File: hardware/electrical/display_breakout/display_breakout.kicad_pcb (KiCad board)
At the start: 2 copper layers, 4 parts, among them J1 Conn_02x10_Odd_Even, SW1 RotaryEncoder_Switch, SW2 SW_Push, SW3 SW_Push

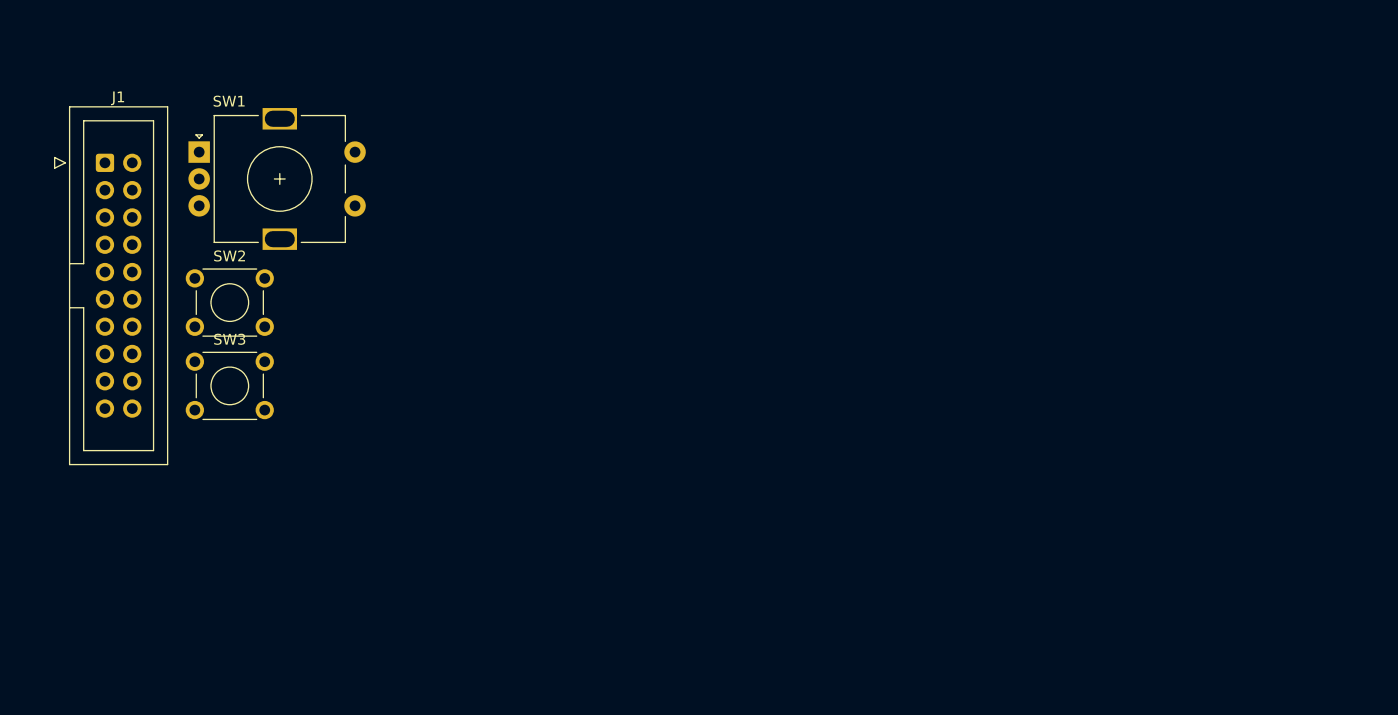
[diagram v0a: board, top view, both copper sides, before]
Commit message: updated schematic to latest version
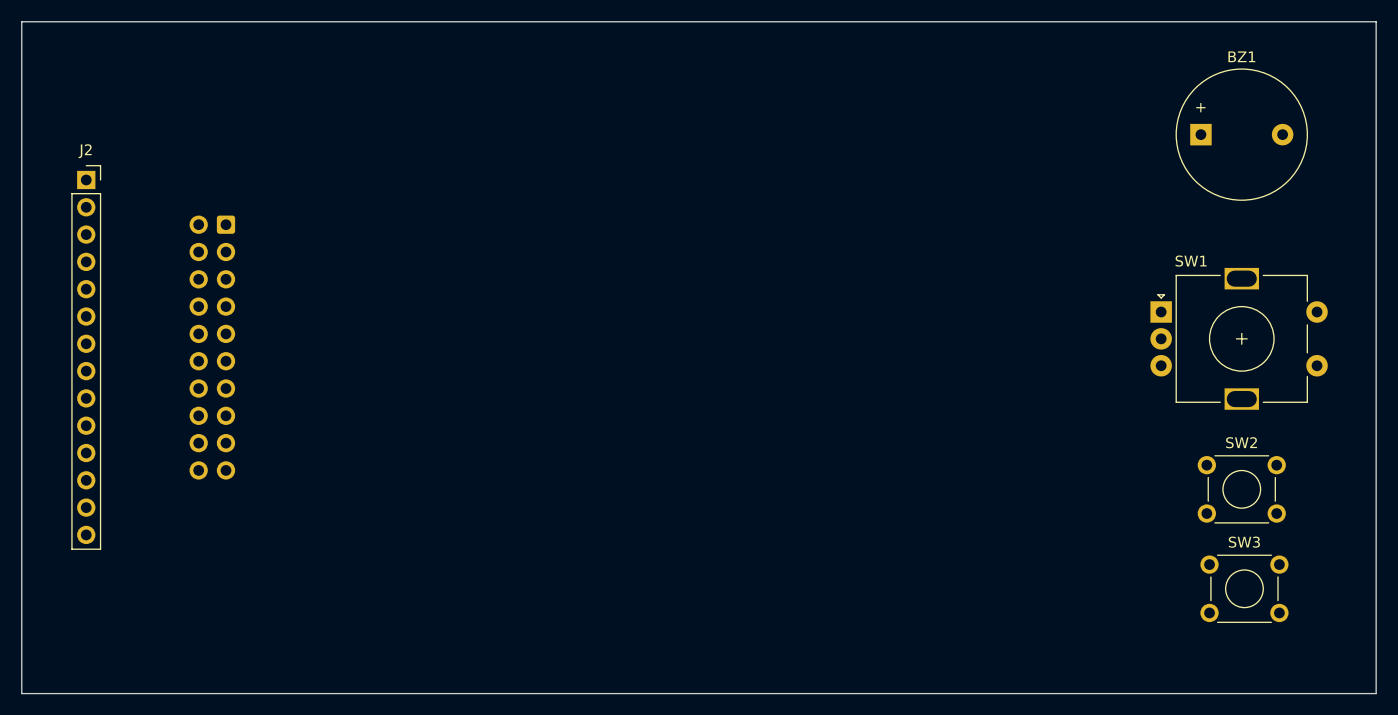
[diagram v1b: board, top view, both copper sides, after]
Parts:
- added BZ1: Buzzer, Buzzer_Beeper:Buzzer_12x9.5RM7.6, F.Cu at (221.7, 64.0)
- added J2: Conn_01x14_Socket, Connector_PinSocket_2.54mm:PinSocket_1x14_P2.54mm_Vertical, F.Cu at (118.0, 68.2)
- J1: moved to B.Cu
- moved SW3 96.3 mm to (222.5, 104.0)
- moved SW2 95.7 mm to (222.2, 94.8)
- moved SW1 90.7 mm to (218.0, 80.5)
- moved J1 12.6 mm to (131.0, 72.4), turned to 180 degrees
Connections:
- J1 pad 12: /SPI_MOSI -> /TOUCH_IRQ
- J1 pad 14: /TOUCH_IRQ -> /EC11_B (DT)
- J1 pad 16: /EC11_B (DT) -> /BTN1
- J1 pad 18: /BTN1 -> /BUZ_PWM
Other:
- board outline added: 126 x 62.5 mm
